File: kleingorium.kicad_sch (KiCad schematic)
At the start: 18 parts, among them J1 4017 Pins, J10 VCC, J11 GND, J12 4046 Comp In, J2 4040 Output, J3 4040 Input, J4 4046 Out, J5 4046 Comp, J6 Select, J7 Output, J8 Input, J9 4046 SigIn, Q1 2N3904, SW1 4017 Feedback, SW2 4046 CompIn, SW3 Chain

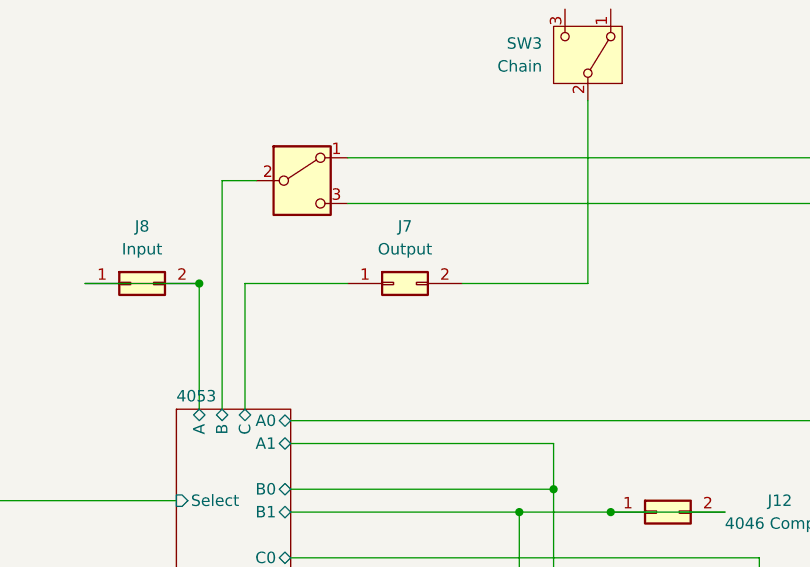
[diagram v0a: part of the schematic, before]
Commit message: after main routing
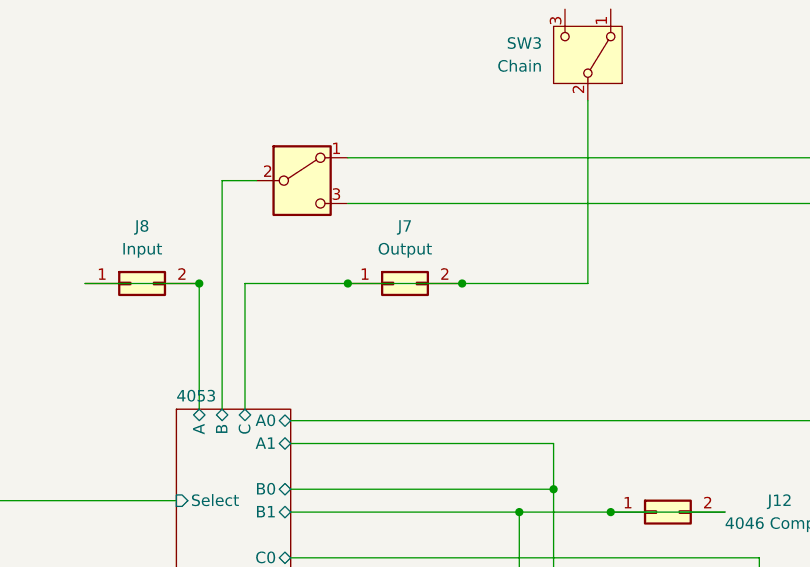
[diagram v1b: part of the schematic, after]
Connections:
- net 4053/C: now also J7.2 (Pin_2), SW3.2 (B)
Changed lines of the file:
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@@
+	)
+	(junction
+		(at 91.44 175.26)
+		(diameter 0)
+		(color 0 0 0 0)
 	)
 	(junction
@@
 	)
 	(junction
+		(at 104.14 175.26)
+		(diameter 0)
+		(color 0 0 0 0)
+	)
+	(junction
 		(at 254 236.22)
 		(diameter 0)
@@
 		)
 		(stroke
+			(width 0)
+			(type default)
+		)
+	)
+	(wire
+		(pts
+			(xy 91.44 175.26) (xy 104.14 175.26)
+		)
+		(stroke
